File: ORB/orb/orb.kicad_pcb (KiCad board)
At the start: 2 copper layers, 124 x 42 mm, 17 parts, among them U1 Arduino_Nano, U3 CD4071

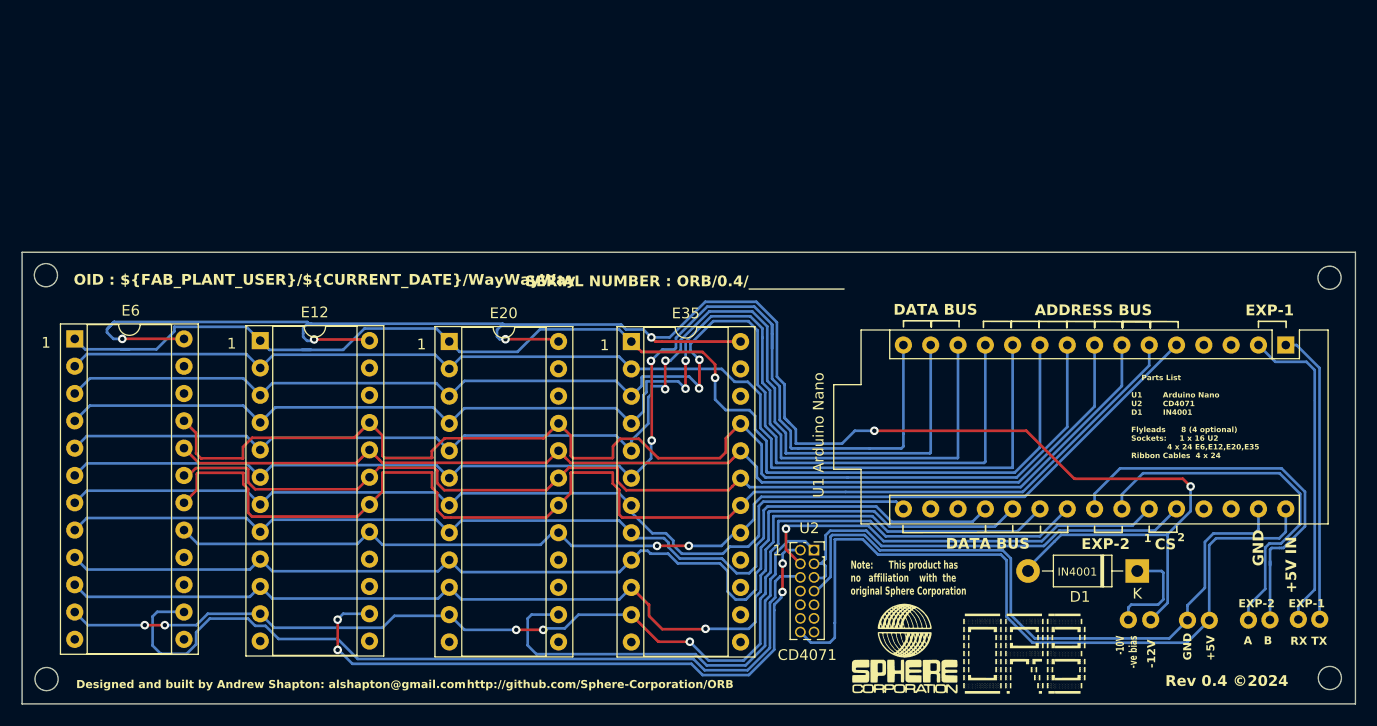
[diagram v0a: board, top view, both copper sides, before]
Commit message: Updated for 0.4.alpha release
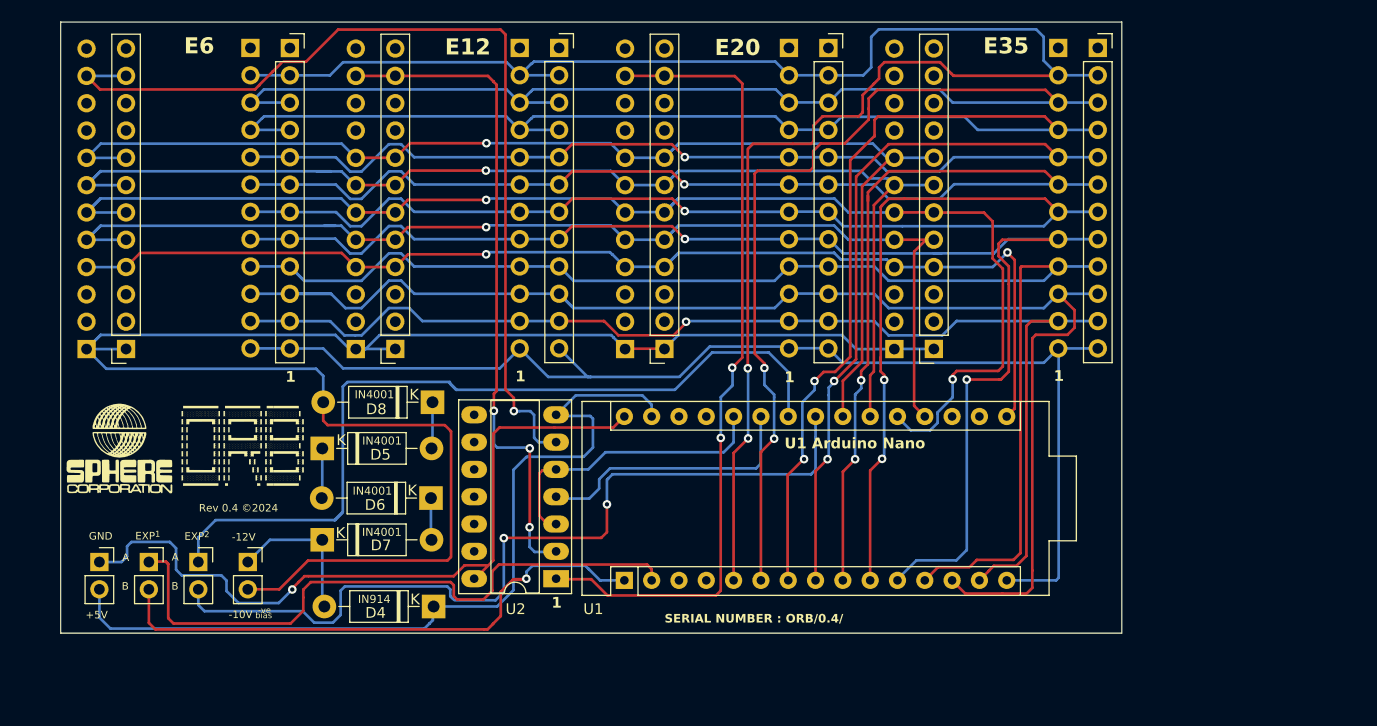
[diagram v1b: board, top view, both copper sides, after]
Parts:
- removed ? (x8): , 
- removed D1: 1N4001, Diode_THT:D_DO-41_SOD81_P10.16mm_Horizontal
- removed E12, E20, E35, E6: MM1702A, Package_DIP:DIP-24_W10.16mm_Socket
- removed U3: CD4071, Connector_PinSocket_1.27mm:PinSocket_2x07_P1.27mm_Vertical
- added D4: IN914, Diode_THT:D_DO-41_SOD81_P10.16mm_Horizontal, F.Cu at (128.3, 78.9)
- added D5: IN4001, Diode_THT:D_DO-41_SOD81_P10.16mm_Horizontal, F.Cu at (117.9, 64.2)
- added D6: IN4001, Diode_THT:D_DO-41_SOD81_P10.16mm_Horizontal, F.Cu at (128.0, 68.9)
- added D7: IN4001, Diode_THT:D_DO-41_SOD81_P10.16mm_Horizontal, F.Cu at (117.9, 72.7)
- added D8: IN4001, Diode_THT:D_DO-41_SOD81_P10.16mm_Horizontal, F.Cu at (128.2, 59.9)
- added E12-1: Conn_01x12_Pin, Connector_PinHeader_2.54mm:PinHeader_1x12_P2.54mm_Vertical, B.Cu at (121.0, 55.0)
- added E12-2: Conn_01x12_Pin, Connector_PinHeader_2.54mm:PinHeader_1x12_P2.54mm_Vertical, B.Cu at (136.3, 27.0)
- added E12-3: Conn_01x12_Pin, Connector_PinSocket_2.54mm:PinSocket_1x12_P2.54mm_Vertical, F.Cu at (124.7, 55.0)
- added E12-4: Conn_01x12_Pin, Connector_PinSocket_2.54mm:PinSocket_1x12_P2.54mm_Vertical, F.Cu at (139.9, 27.0)
- added E20-1: Conn_01x12_Pin, Connector_PinHeader_2.54mm:PinHeader_1x12_P2.54mm_Vertical, B.Cu at (146.1, 55.0)
- added E20-2: Conn_01x12_Pin, Connector_PinHeader_2.54mm:PinHeader_1x12_P2.54mm_Vertical, B.Cu at (161.3, 27.0)
- added E20-3: Conn_01x12_Pin, Connector_PinSocket_2.54mm:PinSocket_1x12_P2.54mm_Vertical, F.Cu at (149.7, 55.0)
- added E20-4: Conn_01x12_Pin, Connector_PinSocket_2.54mm:PinSocket_1x12_P2.54mm_Vertical, F.Cu at (165.0, 27.0)
- added E35-1: Conn_01x12_Pin, Connector_PinHeader_2.54mm:PinHeader_1x12_P2.54mm_Vertical, B.Cu at (171.1, 55.0)
- added E35-2: Conn_01x12_Pin, Connector_PinHeader_2.54mm:PinHeader_1x12_P2.54mm_Vertical, B.Cu at (186.4, 27.0)
- added E35-3: Conn_01x12_Pin, Connector_PinSocket_2.54mm:PinSocket_1x12_P2.54mm_Vertical, F.Cu at (174.8, 55.0)
- added E35-4: Conn_01x12_Pin, Connector_PinSocket_2.54mm:PinSocket_1x12_P2.54mm_Vertical, F.Cu at (190.0, 27.0)
- added E6-1: E6-1C, Connector_PinHeader_2.54mm:PinHeader_1x12_P2.54mm_Vertical, B.Cu at (96.0, 55.0)
- added E6-2: Conn_01x12_Pin, Connector_PinHeader_2.54mm:PinHeader_1x12_P2.54mm_Vertical, B.Cu at (111.2, 27.0)
- added E6-3: E6-1C, Connector_PinSocket_2.54mm:PinSocket_1x12_P2.54mm_Vertical, F.Cu at (99.7, 55.0)
- added E6-4: Conn_01x12_Pin, Connector_PinSocket_2.54mm:PinSocket_1x12_P2.54mm_Vertical, F.Cu at (114.9, 27.0)
- added J1: Conn_01x02_Socket, Connector_PinSocket_2.54mm:PinSocket_1x02_P2.54mm_Vertical, F.Cu at (97.2, 74.8)
- added J2: Conn_01x02_Socket, Connector_PinSocket_2.54mm:PinSocket_1x02_P2.54mm_Vertical, F.Cu at (101.8, 74.8)
- added J3: Conn_01x02_Socket, Connector_PinSocket_2.54mm:PinSocket_1x02_P2.54mm_Vertical, F.Cu at (106.4, 74.8)
- added J4: Conn_01x02_Socket, Connector_PinSocket_2.54mm:PinSocket_1x02_P2.54mm_Vertical, F.Cu at (111.0, 74.8)
- added U2: 4071, Package_DIP:DIP-14_W7.62mm_Socket_LongPads, F.Cu at (139.7, 76.4)
- moved G*** 75.4 mm to (99.1, 64.2)
- moved G*** 75.2 mm to (110.6, 64.4)
- moved U1 65.3 mm to (146.0, 76.5), turned to 90 degrees
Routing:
- net Net-(D1-A): track 178.3 -> 0.00 mm, vias 6 -> 0
- net Net-(D8-A): track 0.00 -> 162.6 mm
- net Net-(E6-1-Pin_11): track 0.00 -> 87.1 mm, vias 0 -> 1
- net Net-(E6-~{CS}): track 77.4 -> 0.00 mm
- net Net-(E20-1-Pin_11): track 0.00 -> 75.4 mm, vias 0 -> 2
- net Net-(E12-2-Pin_2): track 103.3 -> 166.9 mm
- net Net-(E12-1-Pin_11): track 0.00 -> 62.2 mm, vias 0 -> 3
- net Net-(E12-~{CS}): track 59.5 -> 0.00 mm, vias 4 -> 0
- net Net-(E12-2-Pin_4): track 102.4 -> 154.0 mm, vias 0 -> 2
- net Net-(E12-2-Pin_3): track 116.0 -> 162.3 mm, vias 0 -> 2
- net Net-(E12-2-Pin_5): track 98.1 -> 142.7 mm, vias 0 -> 3
- net Net-(J3-Pin_1): track 33.9 -> 78.5 mm
- net Net-(E20-~{CS}): track 42.5 -> 0.00 mm
- net Net-(J3-Pin_2): track 36.5 -> 78.8 mm, vias 0 -> 2
- net Net-(J2-Pin_1): track 29.9 -> 59.9 mm
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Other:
- board size 124 x 42 mm -> 98.7 x 56.8 mm
- board text added: "-10V"
- board text added: "A"
- board text added: "B"
- board text added: "E12"
- board text added: "E20"
- board text added: "E35"
- board text added: "E6"
- board text added: "EXP^{1}"
- board text added: "EXP^{2}"
- board text added: "IN914"
- board text added: "SERIAL NUMBER : ORB/0.4/"
- board text added: "U1"
- board text added: "^{-ve}"
- board text added: "^{bias}"
- board text added: "http://github.com/Sphere-Corporation"
- board text removed: "+5V IN"
- board text removed: "-10V -ve bias"
- board text removed: "2"
- board text removed: "A B"
- board text removed: "ADDRESS BUS"
- board text removed: "CS"
- board text removed: "D1"
- board text removed: "DATA BUS"
- board text removed: "EXP-1"
- board text removed: "EXP-2"
- board text removed: "Parts List U1 Arduino Nano U2 CD4071 D1 IN4001 Flyleads 8 (4 optional) Sockets: 1 x 16 U2 4 x 24 E6,E12,E20,E35 Ribbon Cables 4 x 24"
- board text removed: "RX TX"
- board text removed: "SERIAL NUMBER : ORB/0.4/_____________"
- board text removed: "http://github.com/Sphere-Corporation/ORB"
